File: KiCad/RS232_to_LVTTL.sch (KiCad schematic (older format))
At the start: 15 parts, among them J1 DB25_Female, J2 Conn_01x05, U1 TPS54308, U2 MAX3232

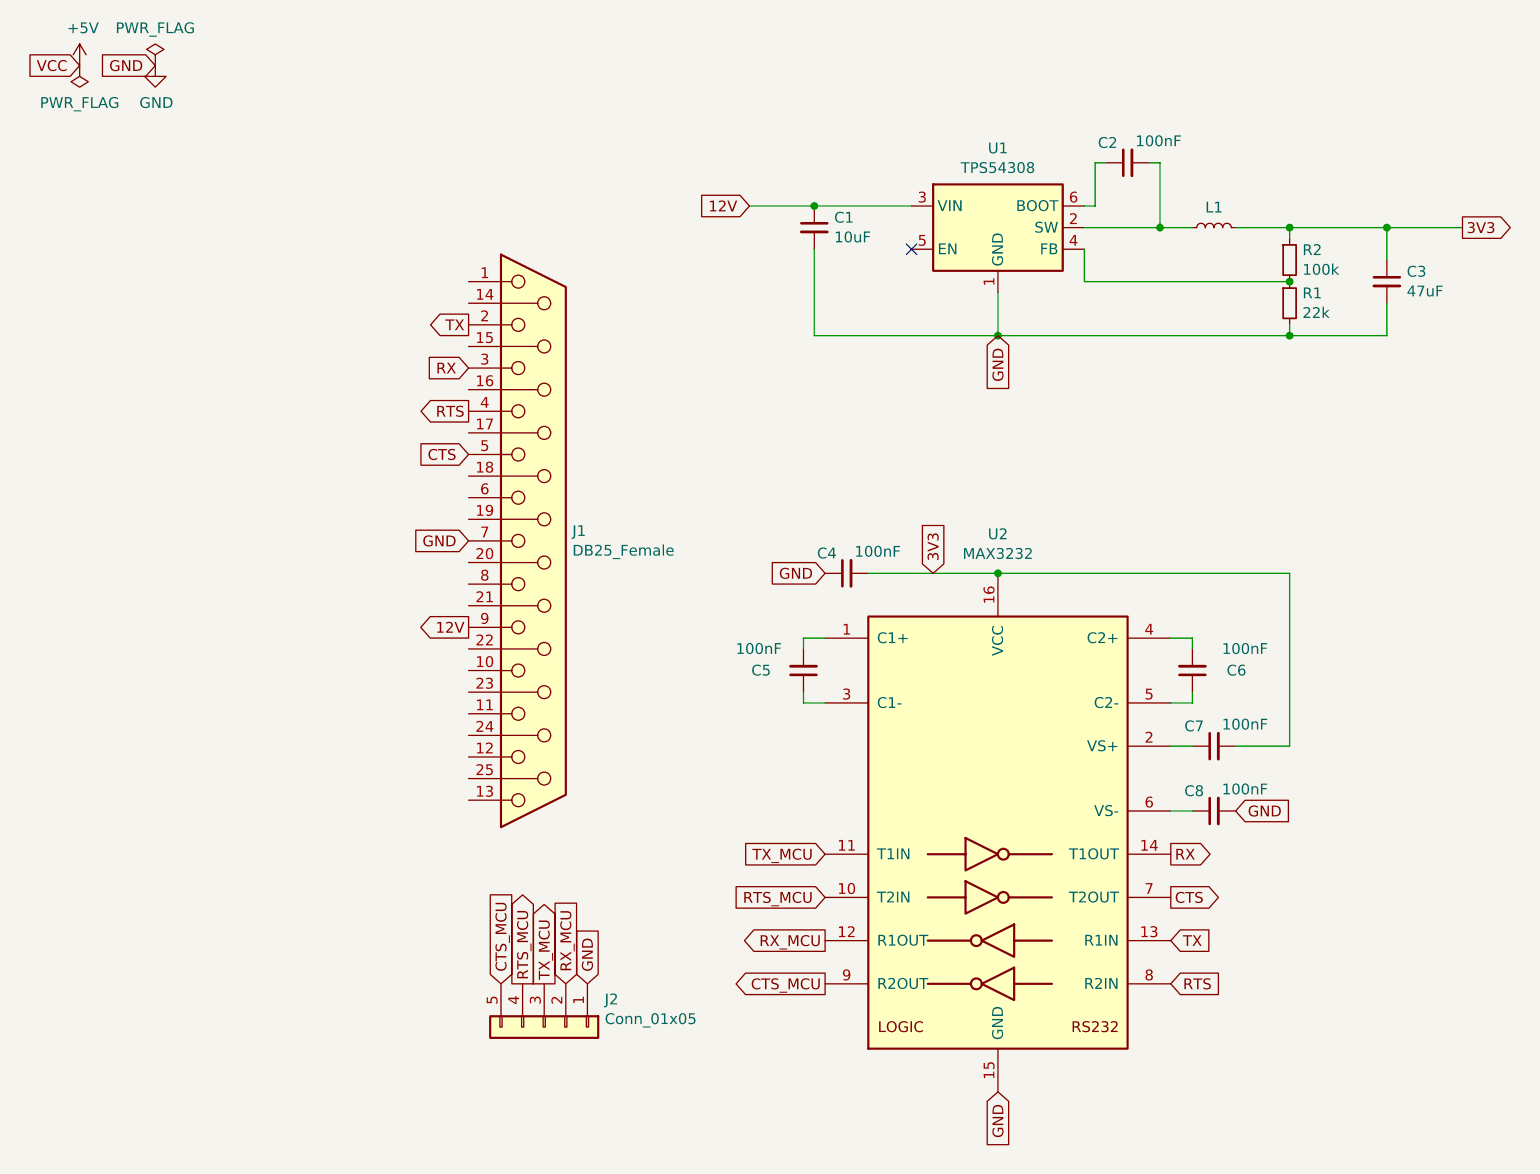
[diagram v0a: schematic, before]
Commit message: routing and placing of components
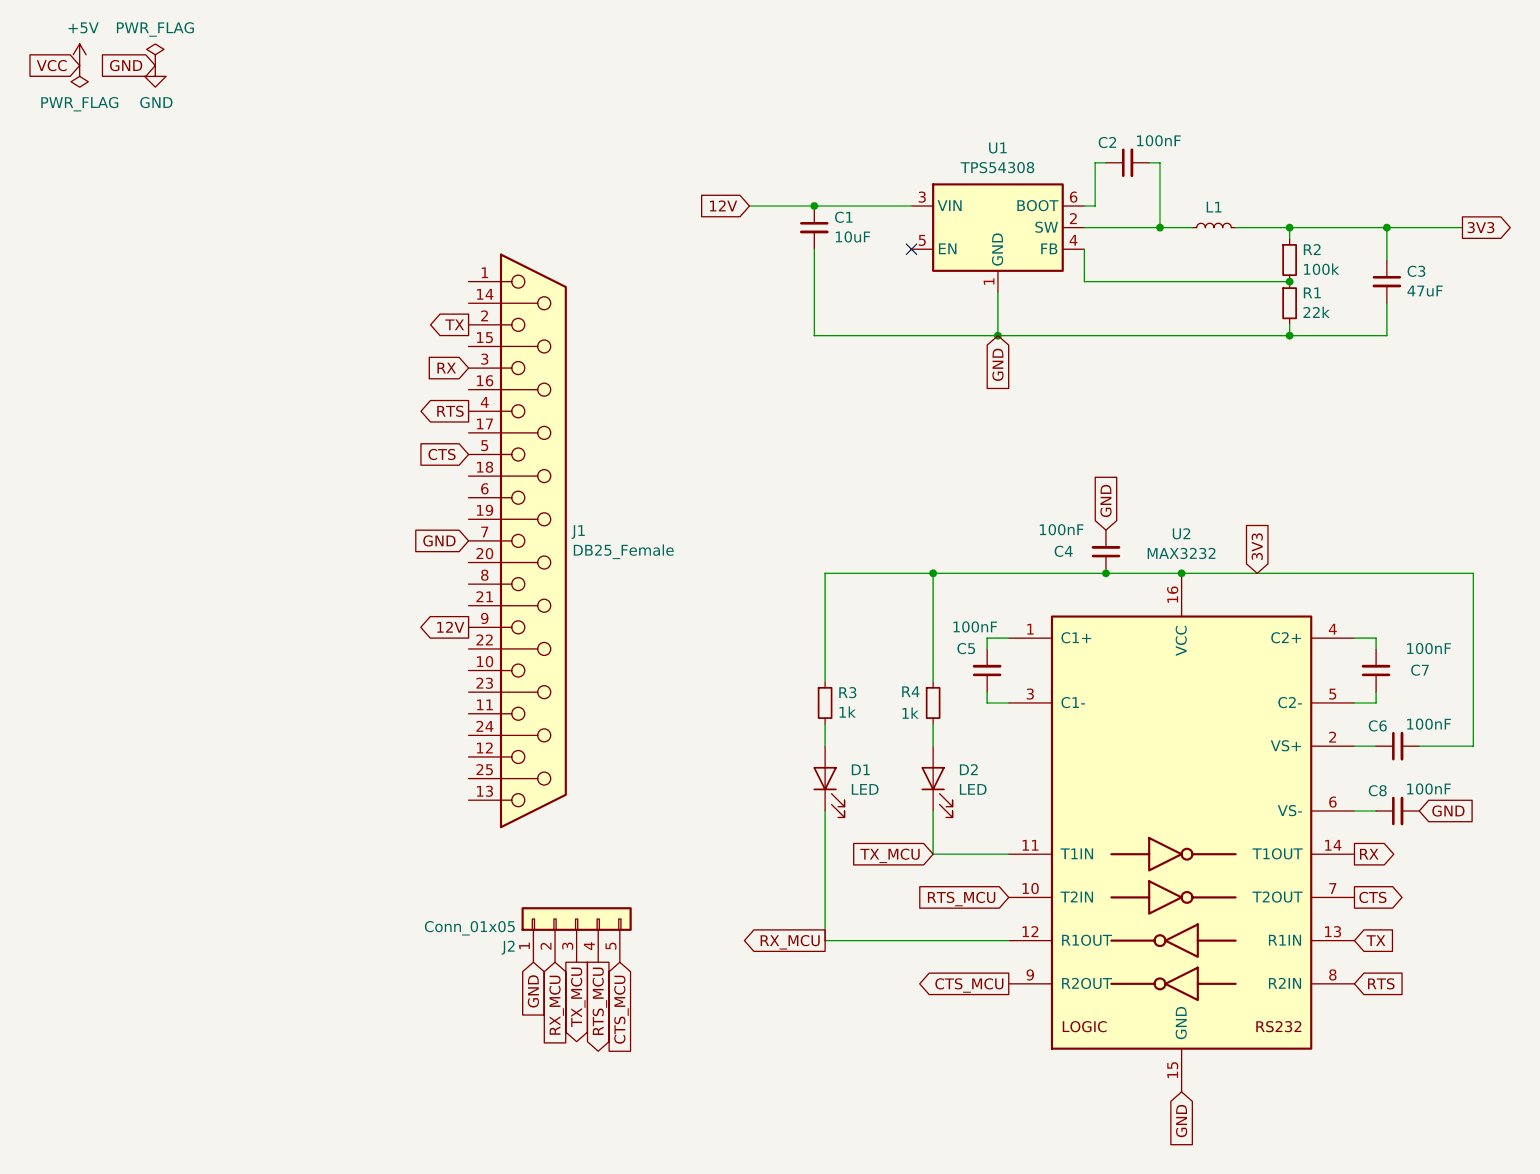
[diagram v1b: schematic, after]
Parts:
- added D1, D2: LED, Diode_SMD:D_0603_1608Metric_Pad1.05x0.95mm_HandSolder, symbol Device:LED
- added R3, R4: 1k, Resistor_SMD:R_0603_1608Metric_Pad1.05x0.95mm_HandSolder, symbol Device:R_Small
- renumbered C7 to C6, C6 to C7
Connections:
- net 3V3: now also C4.1, R3.1, R4.1; no longer C4.2
- net GND: now also C4.2; no longer C4.1
- net RX_MCU: now also D1.1 (K)
- net TX_MCU: now also D2.1 (K)
- new net: D2.2 (A), R4.2
- new net: D1.2 (A), R3.2
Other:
- moved on the sheet: C4, C5, C6, C7, C8, J2, U2
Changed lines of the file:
@@
 L Interface_UART:MAX3232 U2
 U 1 1 64282C45
-P 5200 4500
-F 0 "U2" H 5200 5881 50  0000 C CNN
-F 1 "MAX3232" H 5200 5790 50  0000 C CNN
-F 2 "Package_SO:TSSOP-16_4.4x5mm_P0.65mm" H 5250 3450 50  0001 L CNN
-F 3 "https://datasheets.maximintegrated.com/en/ds/MAX3222-MAX3241.pdf" H 5200 4600 50  0001 C CNN
-	1    5200 4500
+P 6050 4500
+F 0 "U2" H 6050 5881 50  0000 C CNN
+F 1 "MAX3232" H 6050 5790 50  0000 C CNN
+F 2 "Package_SO:TSSOP-16_4.4x5mm_P0.65mm" H 6100 3450 50  0001 L CNN
+F 3 "https://datasheets.maximintegrated.com/en/ds/MAX3222-MAX3241.pdf" H 6050 4600 50  0001 C CNN
+	1    6050 4500
 	1    0    0    -1
 $EndComp
@@
 L Device:C_Small C4
 U 1 1 6428B97E
-P 4500 3300
-F 0 "C4" V 4592 3346 50  0000 L CNN
-F 1 "100nF" V 4600 3050 50  0000 L CNN
-F 2 "Capacitor_SMD:C_0805_2012Metric_Pad1.15x1.40mm_HandSolder" H 4500 3300 50  0001 C CNN
-F 3 "~" H 4500 3300 50  0001 C CNN
-	1    4500 3300
-	0    -1   -1   0
-$EndComp
-Text GLabel 4900 3300 1    50   Input ~ 0
+P 5700 3200
+F 0 "C4" H 5850 3200 50  0000 L CNN
+F 1 "100nF" H 5800 3100 50  0000 L CNN
+F 2 "Capacitor_SMD:C_0805_2012Metric_Pad1.15x1.40mm_HandSolder" H 5700 3200 50  0001 C CNN
+F 3 "~" H 5700 3200 50  0001 C CNN
+	1    5700 3200
+	-1   0    0    1
+$EndComp
+Text GLabel 6400 3300 1    50   Input ~ 0
 3V3
-Wire Wire Line
-	4600 3300 5200 3300
-Text GLabel 4400 3300 0    50   Input ~ 0
-GND
-Text GLabel 6000 4600 2    50   Output ~ 0
+Text GLabel 5700 3100 1    50   Input ~ 0
+GND
+Text GLabel 6850 4600 2    50   Output ~ 0
 RX
-Text GLabel 6000 5000 2    50   Input ~ 0
+Text GLabel 6850 5000 2    50   Input ~ 0
 TX
-Text GLabel 6000 5200 2    50   Input ~ 0
+Text GLabel 6850 5200 2    50   Input ~ 0
 RTS
-Text GLabel 6000 4800 2    50   Output ~ 0
+Text GLabel 6850 4800 2    50   Output ~ 0
 CTS
-Text GLabel 4400 4600 0    50   Input ~ 0
+Text GLabel 4900 4600 0    50   Input ~ 0
 TX_MCU
 Text GLabel 4400 5000 0    50   Output ~ 0
 RX_MCU
-Text GLabel 4400 4800 0    50   Input ~ 0
+Text GLabel 5250 4800 0    50   Input ~ 0
 RTS_MCU
-Text GLabel 4400 5200 0    50   Output ~ 0
+Text GLabel 5250 5200 0    50   Output ~ 0
 CTS_MCU
-Text GLabel 5200 5700 3    50   Input ~ 0
+Text GLabel 6050 5700 3    50   Input ~ 0
 GND
 $Comp
 L Connector_Generic:Conn_01x05 J2
 U 1 1 6429DBB7
-P 3100 5400
-F 0 "J2" V 2972 5680 50  0000 L CNN
-F 1 "Conn_01x05" V 3063 5680 50  0000 L CNN
-F 2 "Connector_PinHeader_2.54mm:PinHeader_1x05_P2.54mm_Vertical" H 3100 5400 50  0001 C CNN
-F 3 "~" H 3100 5400 50  0001 C CNN
-	1    3100 5400
-	0    1    1    0
-$EndComp
-Text GLabel 2900 5200 1    50   Input ~ 0
+P 3250 4900
+F 0 "J2" V 3122 5180 50  0000 L CNN
+F 1 "Conn_01x05" V 3213 5180 50  0000 L CNN
+F 2 "Connector_PinHeader_2.54mm:PinHeader_1x05_P2.54mm_Vertical" H 3250 4900 50  0001 C CNN
+F 3 "~" H 3250 4900 50  0001 C CNN
+	1    3250 4900
+	0    -1   -1   0
+$EndComp
+Text GLabel 3450 5100 3    50   Input ~ 0
 CTS_MCU
-Text GLabel 3000 5200 1    50   Output ~ 0
+Text GLabel 3350 5100 3    50   Output ~ 0
 RTS_MCU
-Text GLabel 3100 5200 1    50   Output ~ 0
+Text GLabel 3250 5100 3    50   Output ~ 0
 TX_MCU
-Text GLabel 3200 5200 1    50   Input ~ 0
+Text GLabel 3150 5100 3    50   Input ~ 0
 RX_MCU
-Text GLabel 3300 5200 1    50   Input ~ 0
-GND
-$Comp
-L Device:C_Small C7
+Text GLabel 3050 5100 3    50   Input ~ 0
+GND
+$Comp
+L Device:C_Small C6
 U 1 1 642A667C
-P 6200 4100
-F 0 "C7" V 6292 4146 50  0000 L CNN
-F 1 "100nF" V 6300 3850 50  0000 L CNN
-F 2 "Capacitor_SMD:C_0603_1608Metric_Pad1.05x0.95mm_HandSolder" H 6200 4100 50  0001 C CNN
-F 3 "~" H 6200 4100 50  0001 C CNN
-	1    6200 4100
-	0    -1   -1   0
-$EndComp
-Wire Wire Line
-	4400 3600 4300 3600
-Wire Wire Line
-	4300 3600 4300 3650
-Wire Wire Line
-	4400 3900 4300 3900
-Wire Wire Line
-	4300 3900 4300 3850
-Wire Wire Line
-	6000 3600 6100 3600
-Wire Wire Line
-	6100 3600 6100 3650
-Wire Wire Line
-	6000 3900 6100 3900
-Wire Wire Line
-	6100 3900 6100 3850
+P 7050 4100
+F 0 "C6" V 7142 4146 50  0000 L CNN
+F 1 "100nF" V 7150 3850 50  0000 L CNN
+F 2 "Capacitor_SMD:C_0603_1608Metric_Pad1.05x0.95mm_HandSolder" H 7050 4100 50  0001 C CNN
+F 3 "~" H 7050 4100 50  0001 C CNN
+	1    7050 4100
+	0    -1   -1   0
+$EndComp
+Wire Wire Line
+	5250 3600 5150 3600
+Wire Wire Line
+	5150 3600 5150 3650
+Wire Wire Line
+	5250 3900 5150 3900
+Wire Wire Line
+	5150 3900 5150 3850
+Wire Wire Line
+	6850 3600 6950 3600
+Wire Wire Line
+	6950 3600 6950 3650
+Wire Wire Line
+	6850 3900 6950 3900
+Wire Wire Line
+	6950 3900 6950 3850
 $Comp
 L Device:C_Small C8
 U 1 1 642AFA1A
-P 6200 4400
-F 0 "C8" V 6292 4446 50  0000 L CNN
-F 1 "100nF" V 6300 4150 50  0000 L CNN
-F 2 "Capacitor_SMD:C_0603_1608Metric_Pad1.05x0.95mm_HandSolder" H 6200 4400 50  0001 C CNN
-F 3 "~" H 6200 4400 50  0001 C CNN
-	1    6200 4400
+P 7050 4400
+F 0 "C8" V 7142 4446 50  0000 L CNN
+F 1 "100nF" V 7150 4150 50  0000 L CNN
+F 2 "Capacitor_SMD:C_0603_1608Metric_Pad1.05x0.95mm_HandSolder" H 7050 4400 50  0001 C CNN
+F 3 "~" H 7050 4400 50  0001 C CNN
+	1    7050 4400
 	0    -1   -1   0
 $EndComp
@@
 L Device:C_Small C5
 U 1 1 642A7281
-P 4300 3750
-F 0 "C5" H 4450 3750 50  0000 L CNN
-F 1 "100nF" H 4400 3650 50  0000 L CNN
-F 2 "Capacitor_SMD:C_0603_1608Metric_Pad1.05x0.95mm_HandSolder" H 4300 3750 50  0001 C CNN
-F 3 "~" H 4300 3750 50  0001 C CNN
-	1    4300 3750
+P 5150 3750
+F 0 "C5" H 5200 3650 50  0000 L CNN
+F 1 "100nF" H 5100 3550 50  0000 L CNN
+F 2 "Capacitor_SMD:C_0603_1608Metric_Pad1.05x0.95mm_HandSolder" H 5150 3750 50  0001 C CNN
+F 3 "~" H 5150 3750 50  0001 C CNN
+	1    5150 3750
 	-1   0    0    1
 $EndComp
 $Comp
-L Device:C_Small C6
+L Device:C_Small C7
 U 1 1 642AA23A
-P 6100 3750
-F 0 "C6" H 5850 3750 50  0000 L CNN
-F 1 "100nF" H 5750 3650 50  0000 L CNN
-F 2 "Capacitor_SMD:C_0603_1608Metric_Pad1.05x0.95mm_HandSolder" H 6100 3750 50  0001 C CNN
-F 3 "~" H 6100 3750 50  0001 C CNN
-	1    6100 3750
+P 6950 3750
+F 0 "C7" H 6700 3750 50  0000 L CNN
+F 1 "100nF" H 6600 3650 50  0000 L CNN
+F 2 "Capacitor_SMD:C_0603_1608Metric_Pad1.05x0.95mm_HandSolder" H 6950 3750 50  0001 C CNN
+F 3 "~" H 6950 3750 50  0001 C CNN
+	1    6950 3750
 	-1   0    0    1
 $EndComp
 Wire Wire Line
-	6000 4100 6100 4100
-Wire Wire Line
-	6300 4100 6550 4100
-Wire Wire Line
-	6550 4100 6550 3300
-Wire Wire Line
-	6550 3300 5200 3300
-Connection ~ 5200 3300
-Wire Wire Line
-	6000 4400 6100 4400
-Text GLabel 6300 4400 2    50   Input ~ 0
-GND
+	6850 4100 6950 4100
+Wire Wire Line
+	7150 4100 7400 4100
+Wire Wire Line
+	7400 4100 7400 3300
+Wire Wire Line
+	7400 3300 6050 3300
+Connection ~ 6050 3300
+Wire Wire Line
+	6850 4400 6950 4400
+Text GLabel 7150 4400 2    50   Input ~ 0
+GND
+$Comp
+L Device:R_Small R4
+U 1 1 642C12CA
+P 4900 3900
+F 0 "R4" H 4750 3950 50  0000 L CNN
+F 1 "1k" H 4750 3850 50  0000 L CNN
+F 2 "Resistor_SMD:R_0603_1608Metric_Pad1.05x0.95mm_HandSolder" H 4900 3900 50  0001 C CNN
+F 3 "~" H 4900 3900 50  0001 C CNN
+	1    4900 3900
+	1    0    0    -1
+$EndComp
+$Comp
+L Device:R_Small R3
+U 1 1 642C874A
+P 4400 3900
+F 0 "R3" H 4459 3946 50  0000 L CNN
+F 1 "1k" H 4459 3855 50  0000 L CNN
+F 2 "Resistor_SMD:R_0603_1608Metric_Pad1.05x0.95mm_HandSolder" H 4400 3900 50  0001 C CNN
+F 3 "~" H 4400 3900 50  0001 C CNN
+	1    4400 3900
+	1    0    0    -1
+$EndComp
+$Comp
+L Device:LED D2
+U 1 1 642CF70A
+P 4900 4250
+F 0 "D2" V 4939 4133 50  0000 R CNN
+F 1 "LED" V 4848 4133 50  0000 R CNN
+F 2 "Diode_SMD:D_0603_1608Metric_Pad1.05x0.95mm_HandSolder" H 4900 4250 50  0001 C CNN
+F 3 "~" H 4900 4250 50  0001 C CNN
+	1    4900 4250
+	0    -1   -1   0
+$EndComp
+Wire Wire Line
+	5250 4600 4900 4600
+Wire Wire Line
+	4900 4600 4900 4400
+Wire Wire Line
+	4400 5000 5250 5000
+$Comp
+L Device:LED D1
+U 1 1 642D846F
+P 4400 4250
+F 0 "D1" V 4439 4133 50  0000 R CNN
+F 1 "LED" V 4348 4133 50  0000 R CNN
+F 2 "Diode_SMD:D_0603_1608Metric_Pad1.05x0.95mm_HandSolder" H 4400 4250 50  0001 C CNN
+F 3 "~" H 4400 4250 50  0001 C CNN
+	1    4400 4250
+	0    -1   -1   0
+$EndComp
+Wire Wire Line
+	4400 3300 4900 3300
+Wire Wire Line
+	4900 4000 4900 4100
+Wire Wire Line
+	4400 4000 4400 4100
+Wire Wire Line
+	4400 3800 4400 3300
+Wire Wire Line
+	4900 3800 4900 3300
+Connection ~ 4900 3300
+Wire Wire Line
+	4400 4400 4400 5000
+Connection ~ 5700 3300
+Wire Wire Line
+	5700 3300 6050 3300
+Wire Wire Line
+	4900 3300 5700 3300
 $EndSCHEMATC
